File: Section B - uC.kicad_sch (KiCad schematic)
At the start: 9 parts, among them J1 Conn_ARM_SWD_TagConnect_TC203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, U1 ATtiny204-SS

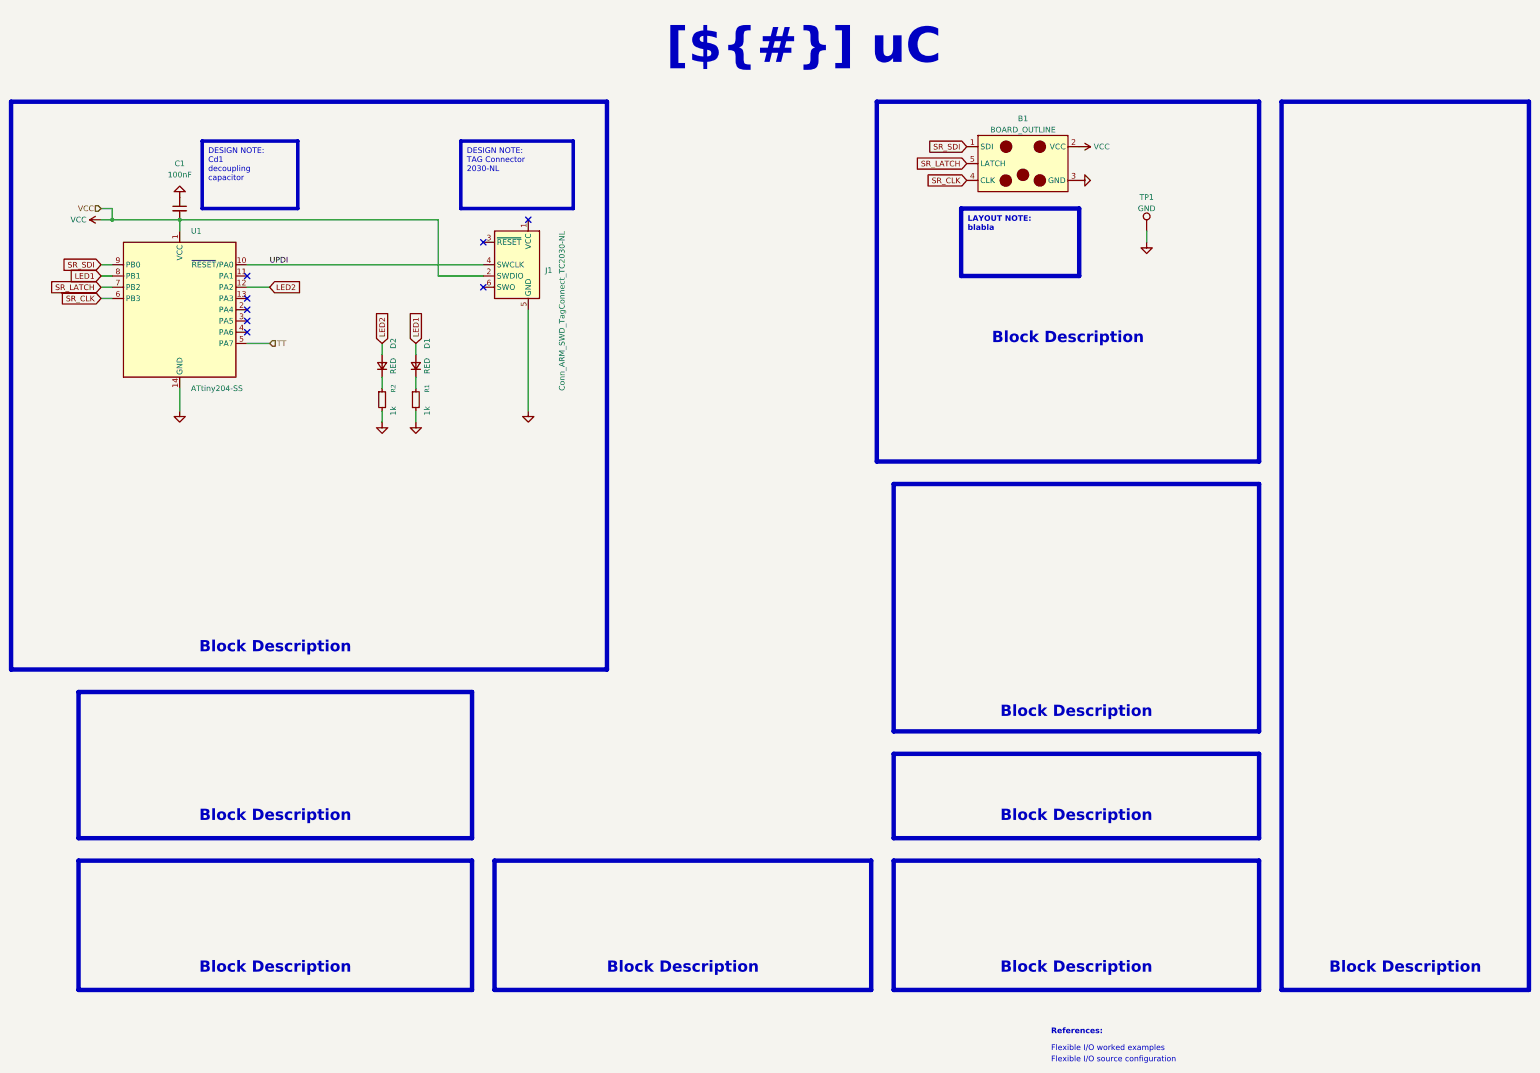
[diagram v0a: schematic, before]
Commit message: touch pad library creation
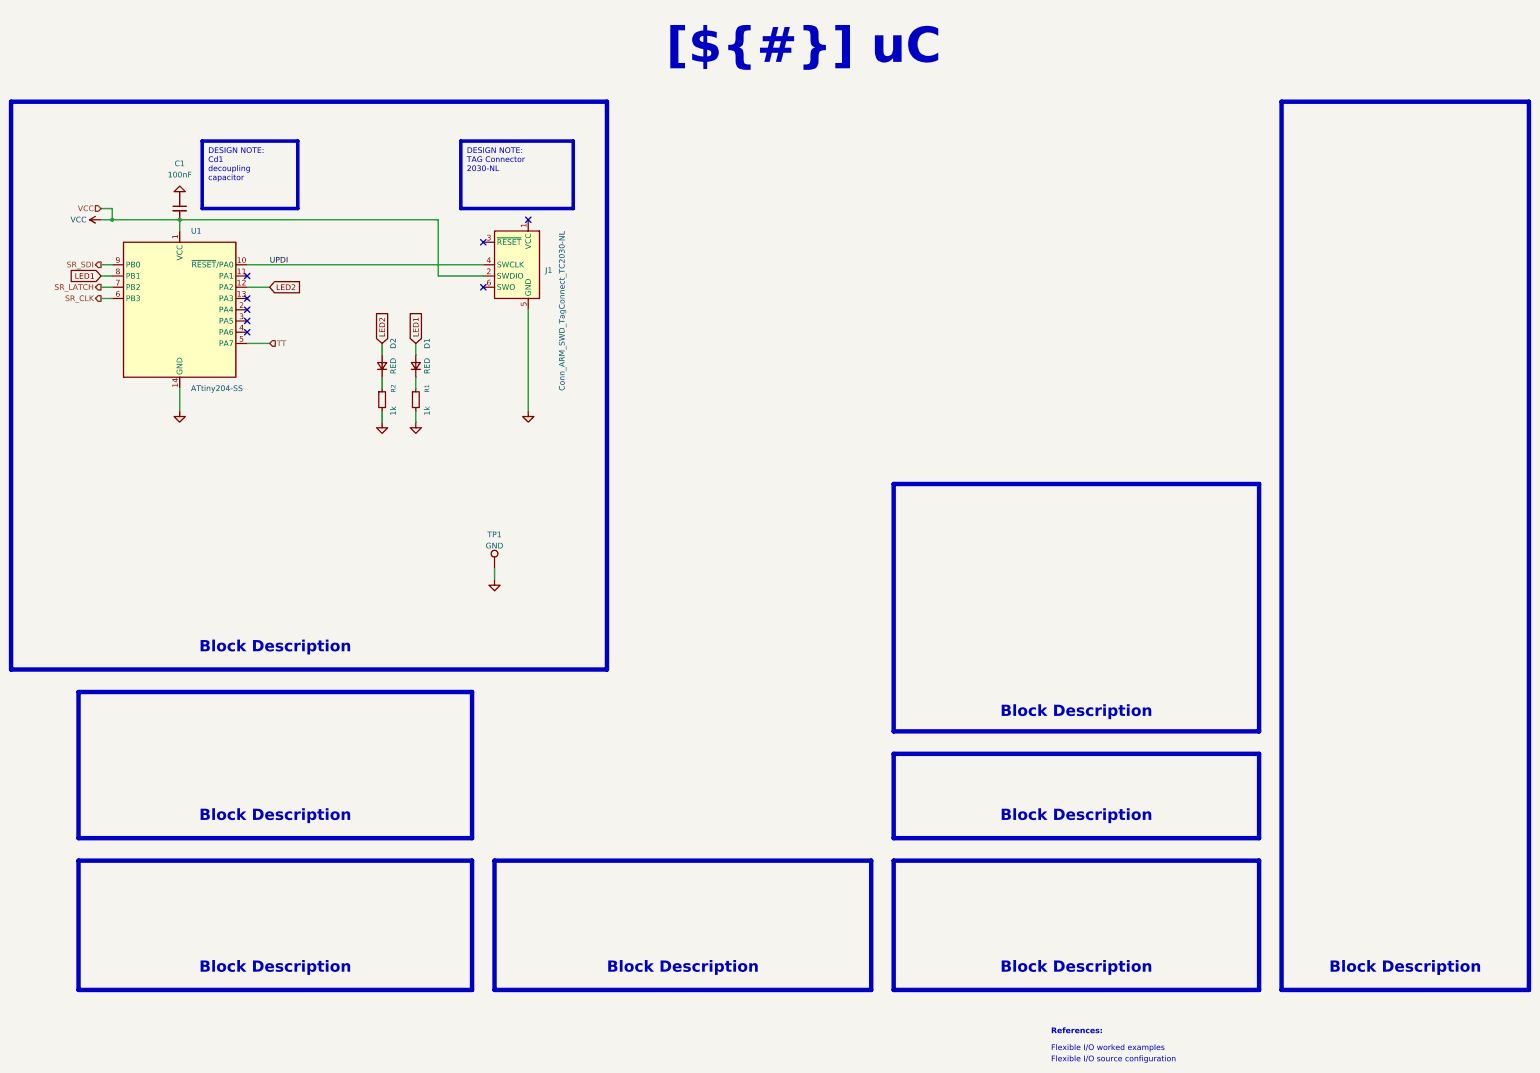
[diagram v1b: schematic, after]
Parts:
- removed B1: BOARD_OUTLINE, __Sienkiewicz:Sienkiewicz, symbol __Sienkiewicz:Sienkiewicz
